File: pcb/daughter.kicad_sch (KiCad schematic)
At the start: 0 parts

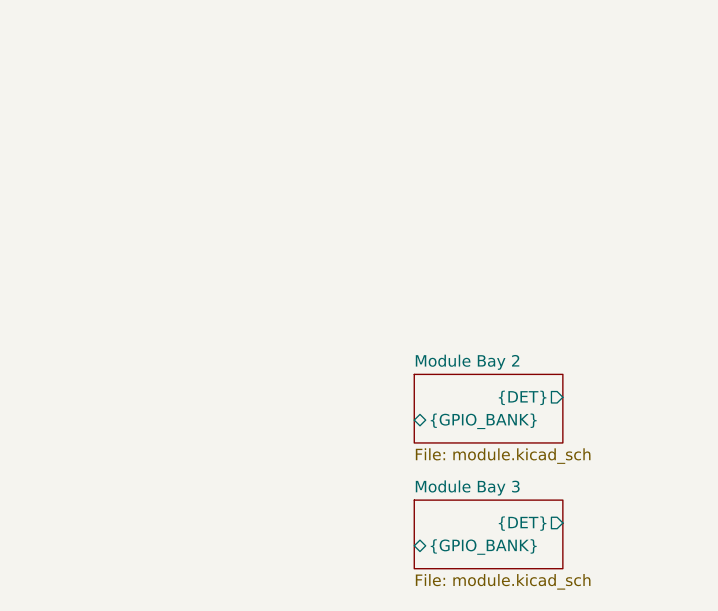
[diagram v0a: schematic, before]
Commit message: moved stuff around
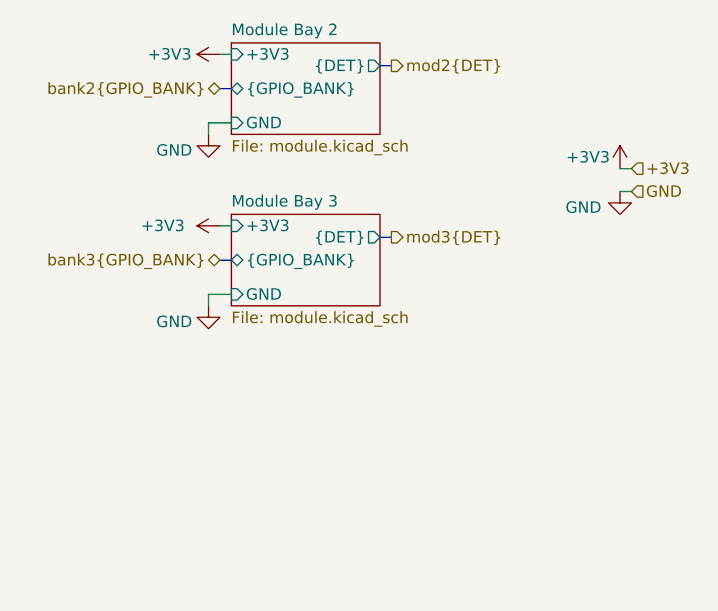
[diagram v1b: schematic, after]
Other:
- sheet Module Bay 2 ports: added +3V3, GND; removed none
- sheet Module Bay 3 ports: added +3V3, GND; removed none
